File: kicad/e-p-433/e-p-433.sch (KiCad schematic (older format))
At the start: 48 parts, among them P1 CONN_01X02, P2 CONN_01X02, P3 Transmitter, P4 ant, P5 Batterie, SW1 SWITCH_INV, SW2 SW_PUSH_m, SW3 Capuchon vert, U1 AD8495ARMZ, U2 AD8495ARMZ, U3 Teensy_3-2, U4 MCP_73831

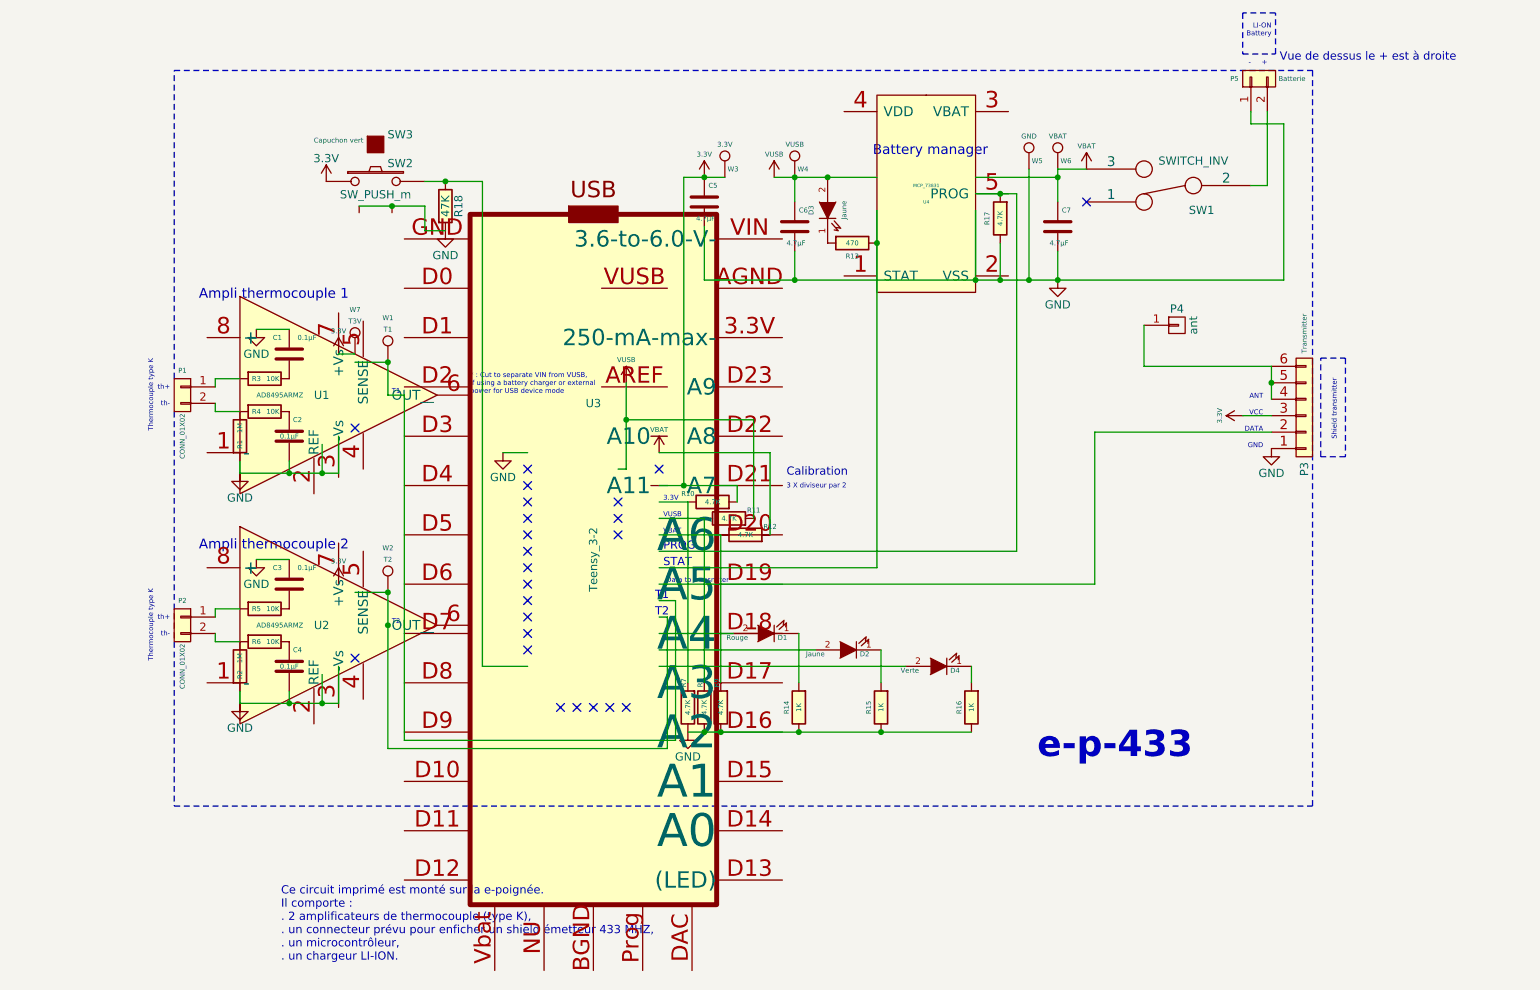
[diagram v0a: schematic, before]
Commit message: Modifier Sp.bak
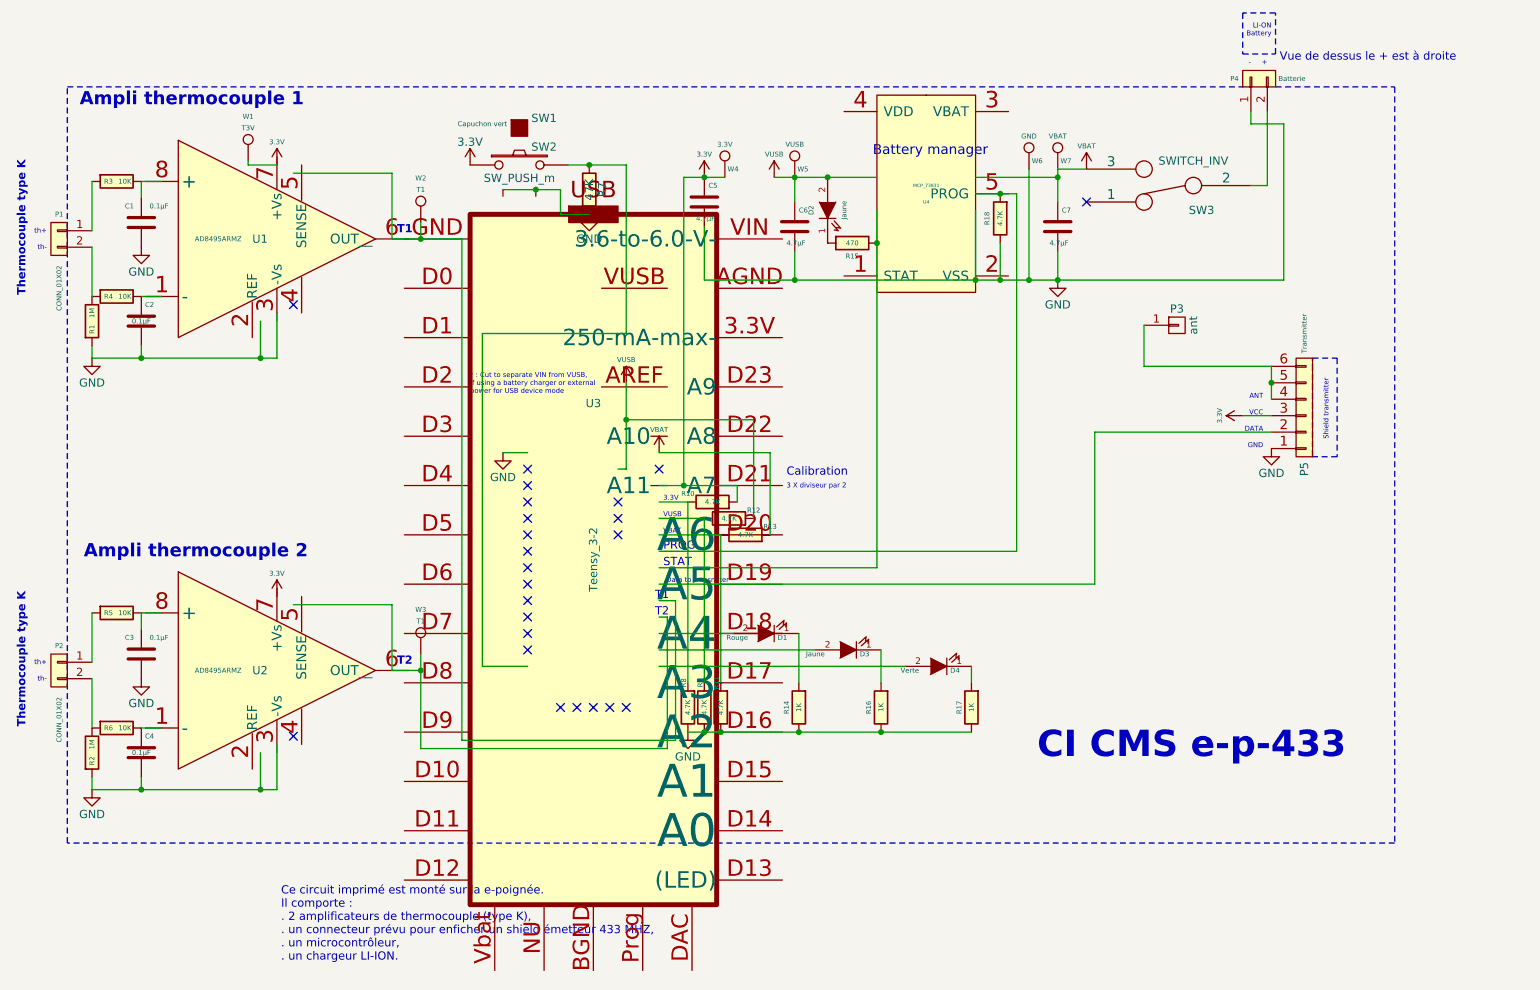
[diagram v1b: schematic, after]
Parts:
- removed W2: T2, Sp:Measurement_Point_Square-SMD-Pad_Big, symbol TEST_1P
- added W3: T1, Sp:Measurement_Point_Square-SMD-Pad_Big, symbol TEST_1P
- renumbered D3 to D2, D2 to D3, P4 to P3, P5 to P4, P3 to P5, R9 to R11, R11 to R12, R12 to R13, R13 to R15, R15 to R16, R16 to R17, R17 to R18, R18 to R7, R7 to R8, R8 to R9, SW3 to SW1, SW1 to SW3, W7 to W1, W1 to W2, W3 to W4, W4 to W5, W5 to W6, W6 to W7
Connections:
- wire segments 92 -> 98
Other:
- note added: "CI CMS e-p-433"
- note removed: "e-p-433"
- moved on the sheet: C1, C2, P1, R1, R3, R4, R7, SW1, SW2, U1, W1, W2
